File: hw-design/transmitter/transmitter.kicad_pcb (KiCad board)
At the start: 2 copper layers, 88 x 36.8 mm, 43 parts, among them P1 CONN_01X03, P10 test-double, P11 test-double, P12 OptionC, P2 test-double, P3 test-double, P4 test-double, P5 test-double, P6 CONN_01X02, P7 test-double, P8 OptionB, P9 OptionA, Q1 2N3904, Q2 2N3904, SW1 power, U1 usb-micro, U2 MCP73833, U3 CD4047, U4 CD4047

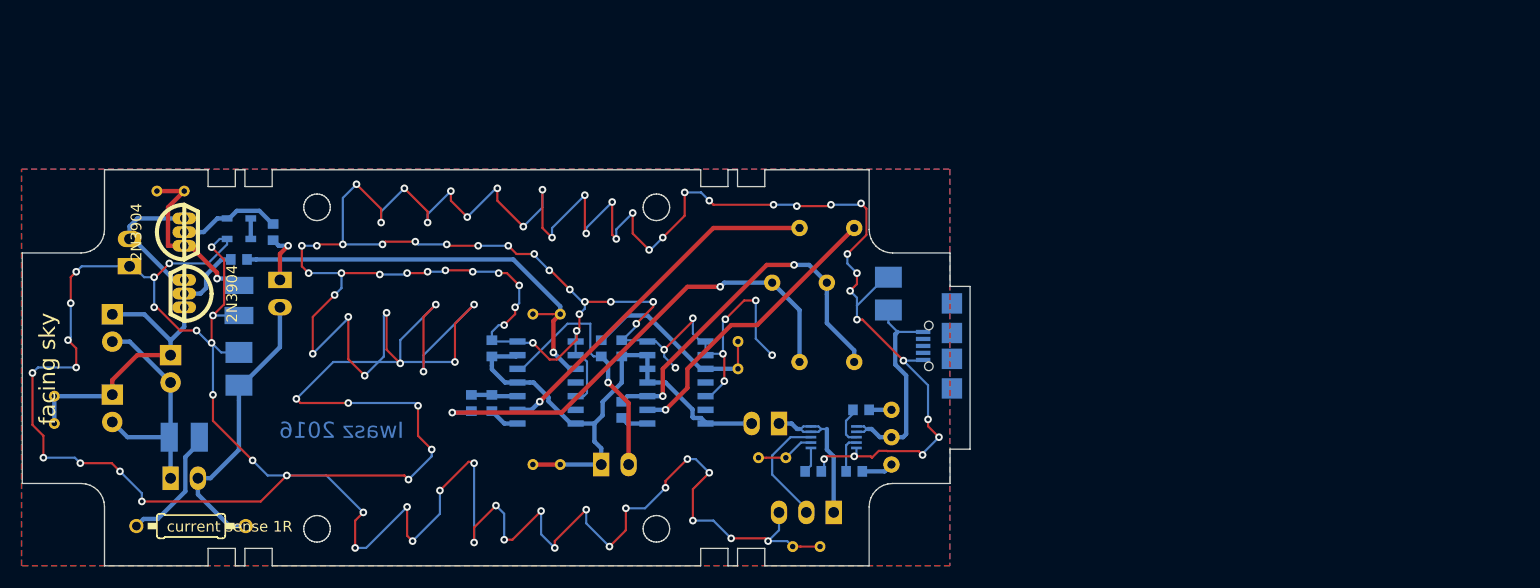
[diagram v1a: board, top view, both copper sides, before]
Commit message: Many changes
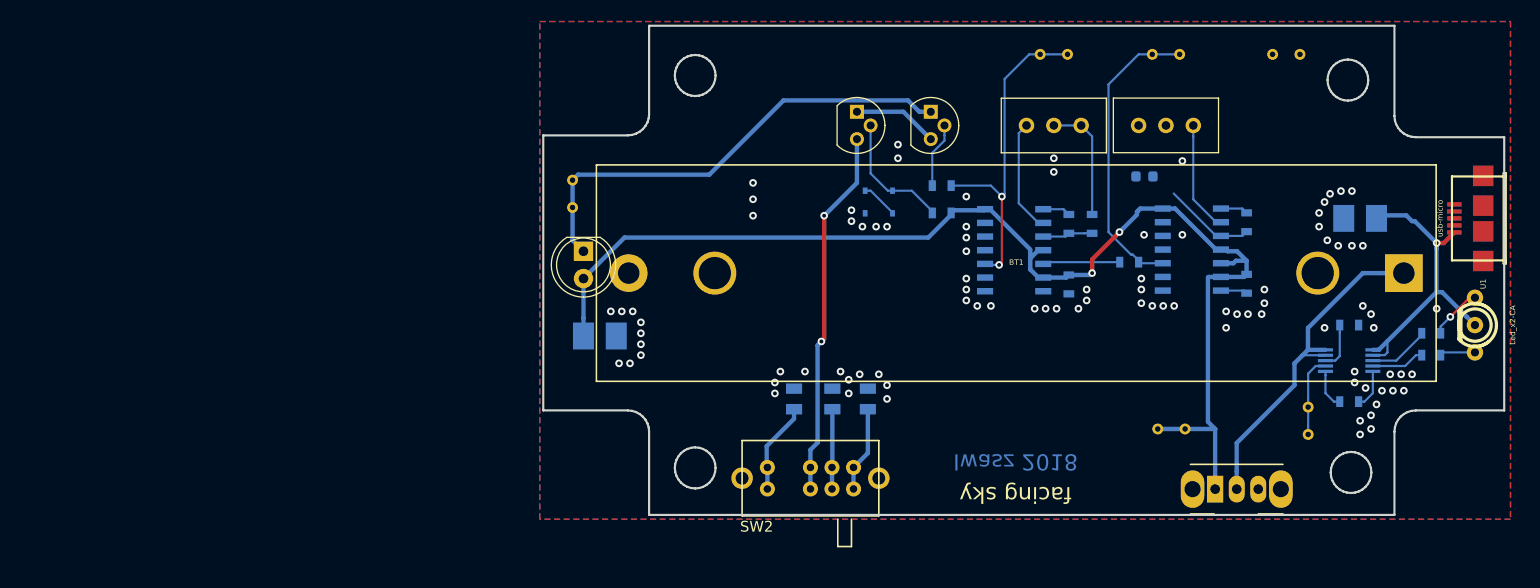
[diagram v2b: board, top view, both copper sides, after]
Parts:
- removed D2, D7: VISHAY TSAL6200, LEDs:LED-5MM
- removed P1: CONN_01X03, w_pin_strip:pin_socket_3
- removed P10: test-double, iwasz:testpad-2p
- removed P12: OptionC, w_pin_strip:pin_socket_2
- removed P6: CONN_01X02, w_pin_strip:pin_socket_2
- removed P8: OptionB, w_pin_strip:pin_socket_2
- removed P9: OptionA, w_pin_strip:pin_socket_2
- added BT1: Battery_Cell, iwasz:BLM-BH18650-PC2, F.Cu at (180.6, 94.0)
- added R10: 4R, Resistor_SMD:R_0805_2012Metric, B.Cu at (127.5, 105.7)
- added R11: 0R, Resistor_SMD:R_0603_1608Metric, B.Cu at (156.5, 85.0)
- added SW2: SW_SP3T, iwasz:switch-3way-8pins-shorted, F.Cu at (125.5, 113.0)
- C2, C3, C4, C5, C6: footprint w_smd_cap:c_0603 -> Capacitor_SMD:C_0603_1608Metric
- D1: moved to F.Cu
- D4: footprint LEDs:LED-5MM -> LED_THT:LED_D5.0mm; moved to F.Cu
- D5, D6: footprint ref-packages:SOD323 -> Diode_SMD:D_SOD-323
- Q1, Q2: footprint w_to:to92_3_flat -> Package_TO_SOT_THT:TO-92
- R1: value 20R -> 10k; footprint w_smd_resistors:r_1210 -> Resistor_SMD:R_0603_1608Metric
- R2, R3, R4, R5, R6, R7: footprint w_smd_resistors:r_0603 -> Resistor_SMD:R_0603_1608Metric
- R8: footprint w_smd_resistors:r_1210 -> Resistor_SMD:R_0805_2012Metric
- R9: value current sense 1R -> 8R; footprint resistor:0207%2f10 -> Resistor_SMD:R_0805_2012Metric; moved to B.Cu
- RV1, RV2: footprint Potentiometers:Potentiometer_Bourns_3006P_Angular_ScrewFront -> Potentiometer_THT:Potentiometer_Bourns_3296W_Vertical; moved to F.Cu
- SW1: footprint w_pin_strip:pin_socket_2 -> Button_Switch_THT:SW_CuK_OS102011MA1QN1_SPDT_Angled; moved to F.Cu
- U1: footprint w_conn_pc:conn_usb_B_micro_smd-2 -> iwasz:conn_usb_B_micro_smd-2-nohole; moved to F.Cu
- U2: footprint ref-packages:MSOP10 -> Package_SSOP:MSOP-10_3x3mm_P0.5mm
- U3, U4: footprint Housings_SOIC:SOIC-14_3.9x8.7mm_Pitch1.27mm -> Package_SOIC:SOIC-14_3.9x8.7mm_P1.27mm
- moved R1 108.7 mm to (175.5, 98.8)
- moved Q1 71.4 mm to (136.7, 79.0)
- moved R6 65.6 mm to (137.7, 85.9), turned to 0 degrees
- moved P3 63.9 mm to (169.7, 73.7), turned to 180 degrees
- moved Q2 63.5 mm to (129.8, 79.0), turned to 270 degrees
- moved R7 62.1 mm to (137.7, 88.4), turned to 180 degrees
- moved D5 60.7 mm to (133.1, 87.4), turned to 90 degrees
- moved C2 60.6 mm to (166.0, 89.3)
- moved R5 60.0 mm to (151.6, 89.4)
- moved R8 59.1 mm to (130.8, 105.7)
- moved C6 58.3 mm to (166.0, 95.0)
- moved D6 58.3 mm to (130.6, 87.4), turned to 90 degrees
- moved P2 58.1 mm to (159.0, 108.5)
- moved R9 57.2 mm to (124.0, 105.7), turned to 270 degrees
- moved C4 56.1 mm to (149.5, 89.4)
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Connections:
- D4 pad 2: Net-(D2-Pad2) -> +BATT
- Q2 pad 3: Net-(P10-Pad1) -> Net-(Q2-Pad3)
- R1 pad 1: Net-(D2-Pad2) -> GND
- R7 pad 1: Net-(P12-Pad1) -> +BATT
- R8 pad 2: Net-(P10-Pad1) -> Net-(R8-Pad2)
- R9 pad 1: Net-(R1-Pad2) -> GND
- R9 pad 2: +BATT -> Net-(R9-Pad2)
- RV1 pad 1: Net-(C2-Pad2) -> Net-(R11-Pad1)
- RV1 pad 2: Net-(C2-Pad2) -> Net-(R11-Pad1)
- SW1 pad 1: Net-(P1-Pad1) -> +BATT
- SW1 pad 2: +BATT -> Net-(BT1-Pad1)
- U1 pad 2: Net-(U1-Pad2) -> (no net)
- U1 pad 3: Net-(U1-Pad3) -> (no net)
- U1 pad 4: Net-(U1-Pad4) -> (no net)
- U2 pad 10: Net-(P1-Pad1) -> Net-(BT1-Pad1)
- U2 pad 8: Net-(P1-Pad2) -> Net-(R1-Pad2)
- U2 pad 9: Net-(P1-Pad1) -> Net-(BT1-Pad1)
- U3 pad 11: Net-(U3-Pad11) -> (no net)
- U3 pad 13: Net-(U3-Pad13) -> (no net)
- U4 pad 11: Net-(U4-Pad11) -> (no net)
- U4 pad 13: Net-(U4-Pad13) -> (no net)
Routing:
- net GND: track 575.9 -> 6.15 mm, vias 124 -> 92
- net +BATT: track 76.9 -> 113.4 mm, vias 0 -> 2
- net Net-(Q2-Pad3): track 0.00 -> 34.3 mm, vias 0 -> 2
- net Net-(R5-Pad1): track 45.0 -> 11.2 mm, vias 2 -> 0
- net Net-(BT1-Pad1): track 0.00 -> 32.5 mm
- net Net-(C2-Pad2): track 34.9 -> 8.56 mm, vias 2 -> 0
- net Net-(RV2-Pad3): track 33.2 -> 10.6 mm, vias 1 -> 0
- net Net-(D2-Pad2): track 21.9 -> 0.00 mm
- net Net-(RV1-Pad3): track 27.2 -> 10.3 mm, vias 1 -> 0
- net Net-(D4-Pad1): track 27.1 -> 43.8 mm
- net Net-(P10-Pad1): track 16.7 -> 0.00 mm, vias 1 -> 0
- net Net-(C3-Pad1): track 23.5 -> 7.18 mm, vias 1 -> 0
- net Net-(P1-Pad1): track 15.1 -> 0.00 mm
- net Net-(P1-Pad2): track 10.9 -> 0.00 mm
- net Net-(C3-Pad2): track 18.2 -> 28.3 mm
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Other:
- board size 88 x 36.8 mm -> 89.3 x 45.4 mm
- net class Default: clearance 0.2032 -> 0.1524
- rule trace_clearance: 0.2032 -> 0.1524
- board text added: "Iwasz 2018"
- board text added: "Obudowa Z45 Kradex"
- board text added: "gnd"
- board text added: "gp8-stopwatch R3"
- board text removed: "-"
- board text removed: "Iwasz 2016"
- board text removed: "complete"
- board text removed: "gp8-stopwatch R2"
- board text removed: "progress"
